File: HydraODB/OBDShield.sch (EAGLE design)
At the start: 10 parts, among them J1 HYDRABUS_SHIELD_CON_HEADER_2X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, J2 HYDRABUS_SHIELD_CON_HEADER_2X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, J3 HYDRABUS_SHIELD_CON_HEADER_2X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, U1 SN65HVD233DG4, U2 SN65HVD233DG4

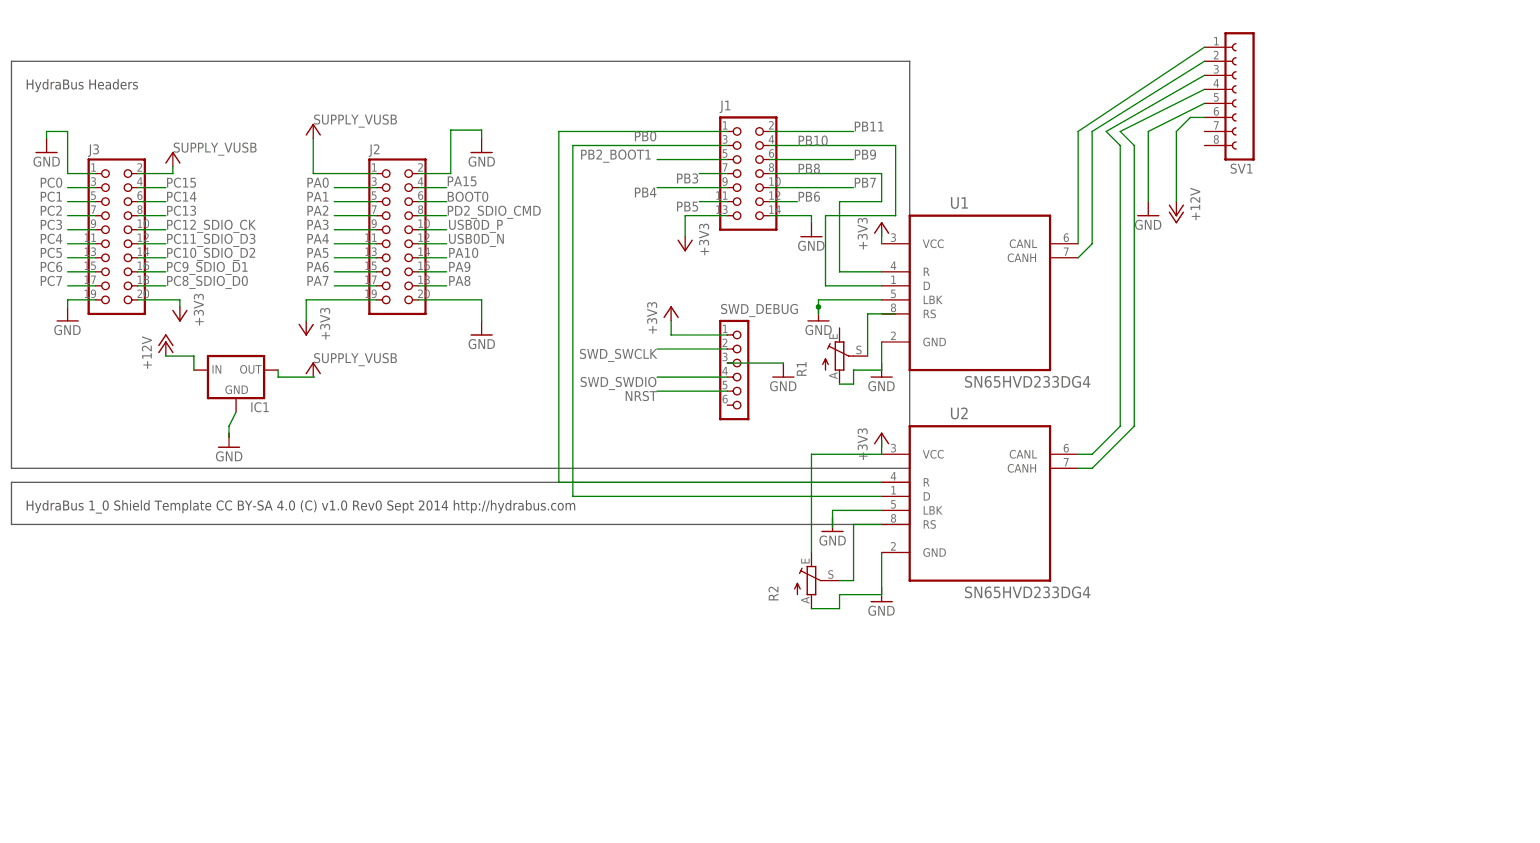
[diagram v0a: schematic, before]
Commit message: Placing and routing
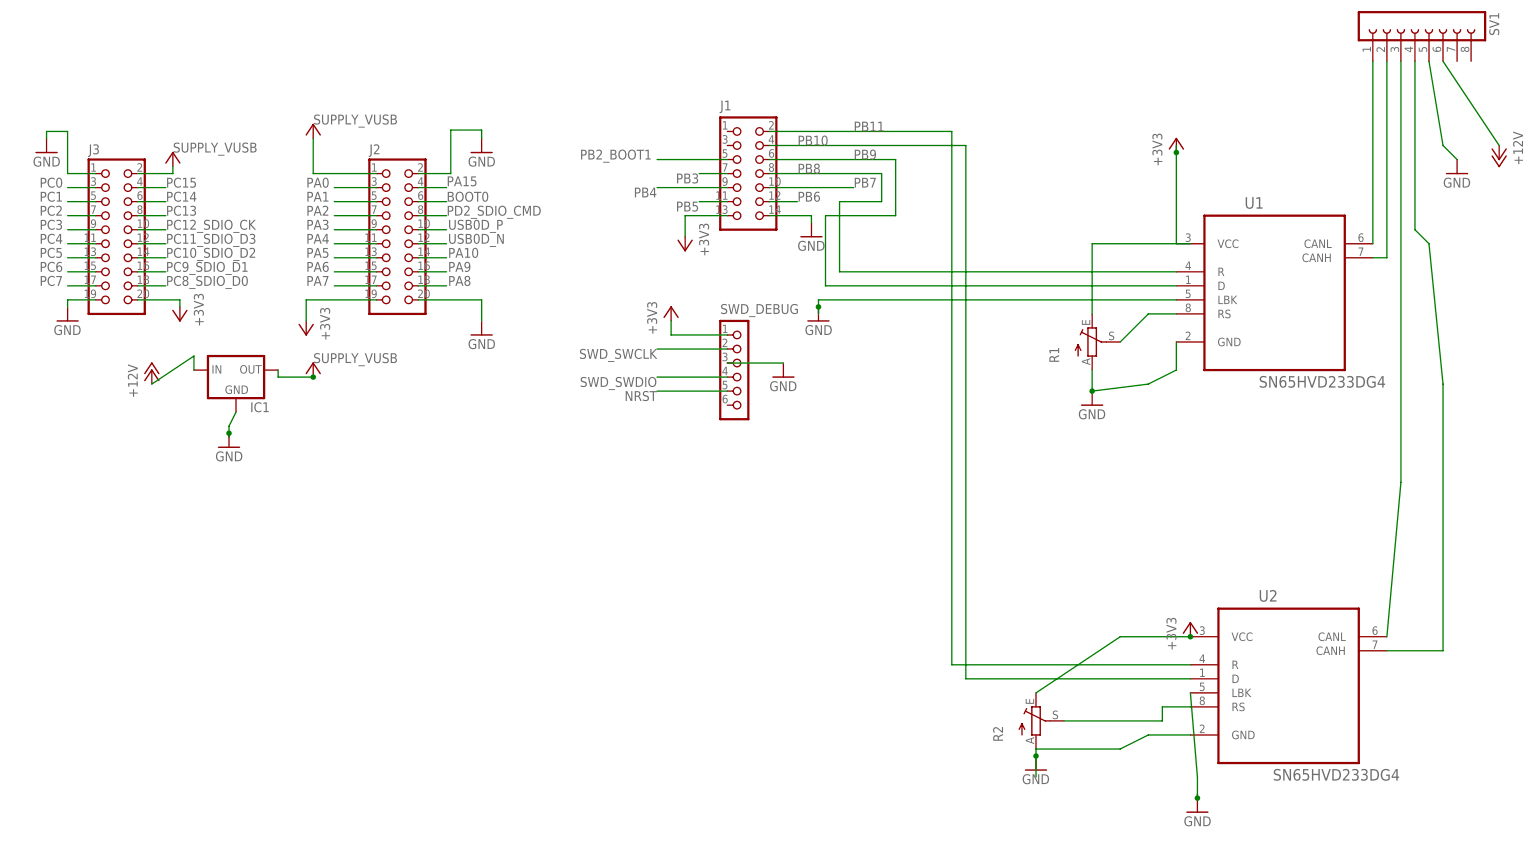
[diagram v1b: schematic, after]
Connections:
- removed net N$13: IC1.GND
- removed net N$14: R2.A, U2.GND
- removed net N$16: R1.S
- removed net N$18: U2.LBK
- removed net N$20: J1.3, U2.D
- removed net N$4: IC1.OUT
- removed net N$6: R2.E, U2.VCC
- removed net N$7: R1.A, U1.GND
- removed net PB0: J1.1, U2.R
- net +3V3: now also R1.E, R2.E, U1.VCC, U2.VCC
- net GND: now also IC1.GND, R1.A, R2.A, U1.GND, U2.GND, U2.LBK
- net N$1: now also R1.S, U1.RS; no longer U1.VCC
- net PB10: now also J1.6; no longer J1.4
- net PB11: now also J1.4, U2.D; no longer J1.2
- net PB9: now also J1.2, U2.R; no longer J1.6
- net VUSB: now also IC1.OUT
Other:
- note removed: "HydraBus 1_0 Shield Template CC BY-SA 4.0 (C) v1.0 Rev0 Sept 2014 http://hydrabus.com"
- note removed: "HydraBus Headers"
- moved on the sheet: R1, R2, SV1, U1, U2
